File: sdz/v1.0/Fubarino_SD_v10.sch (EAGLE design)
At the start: 36 parts, among them IC1 PIC32MZXXXXECX064TQFP-10X10, IC2 MCP1702T-3302E/MB, IC3 DSC1033_MICREL_OSCILLATOR3.2X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, J1 MICRO_SD_CARD_SOCKET, J2 M28USEPIN1, J3 M28NOPIN1, J4 MICRO-USB-5P-340015001, Q2 32.768 KHz

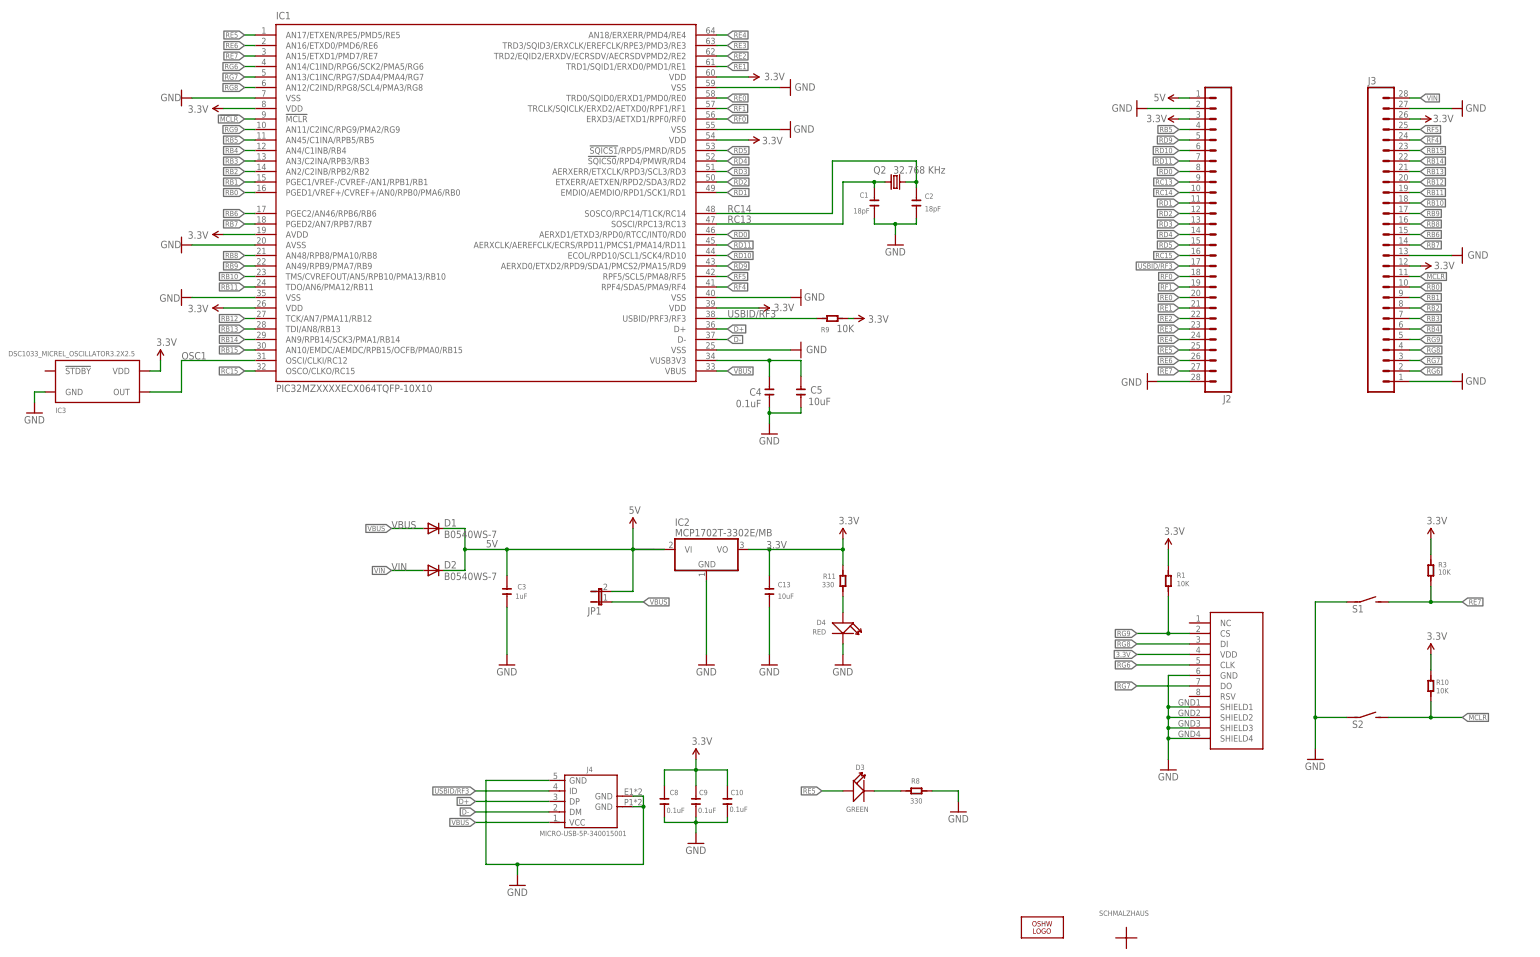
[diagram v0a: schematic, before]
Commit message: This version got sent to seed for fab - v 1.0
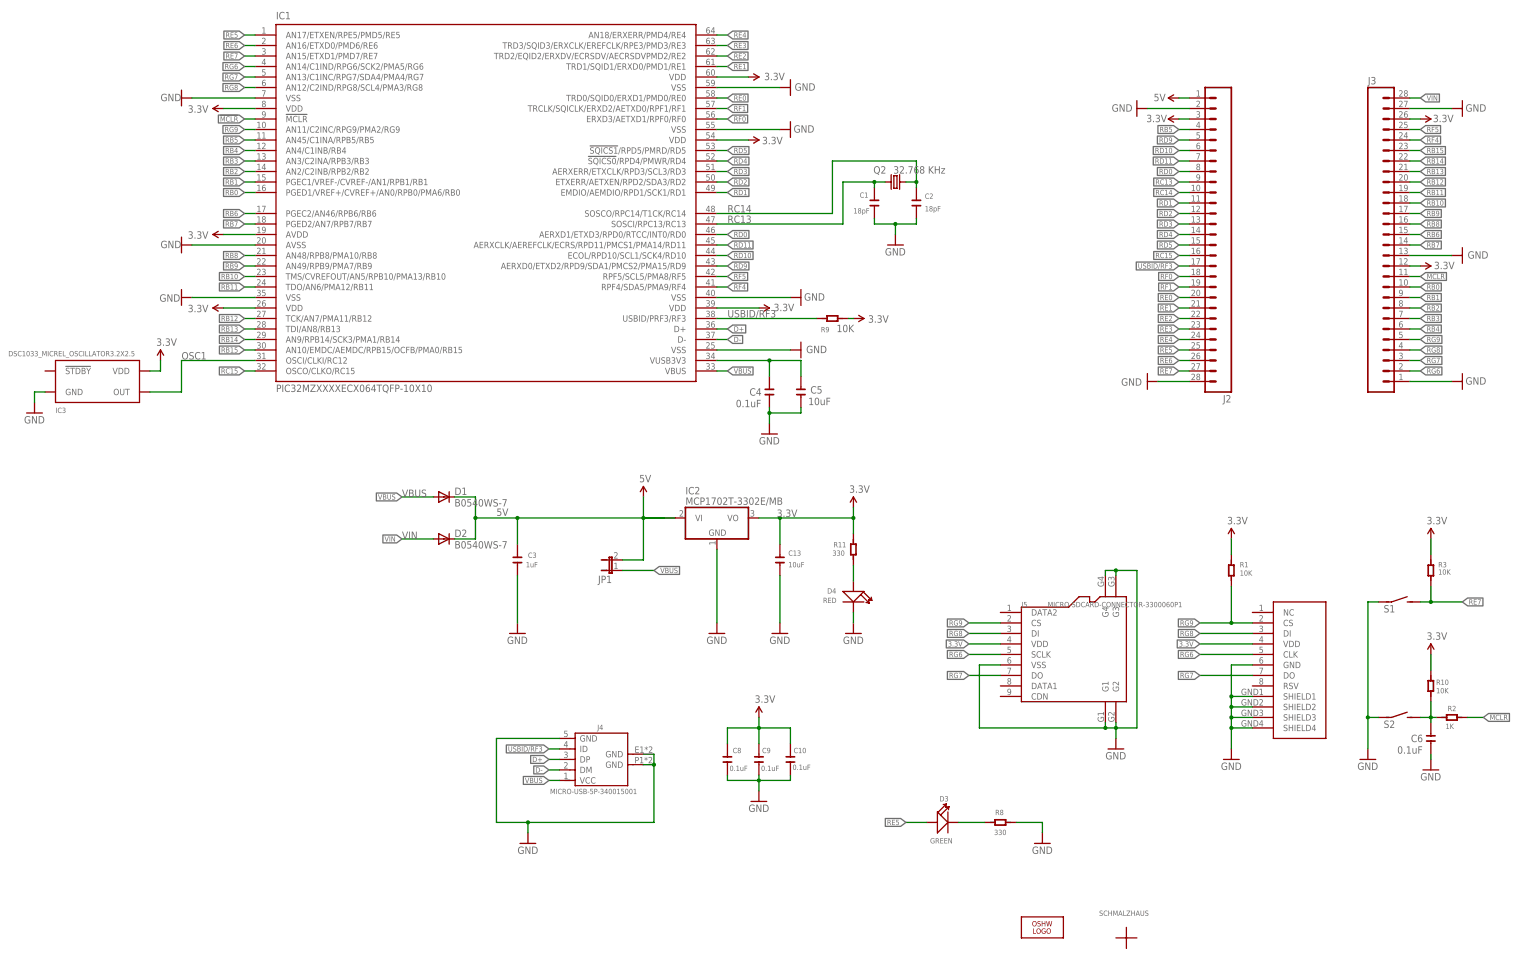
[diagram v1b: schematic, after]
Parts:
- added C6: 0.1uF, OPL Eagle Library:C-0603
- added J5: MICRO-SDCARD-CONNECTOR-3300060P1, OPL Eagle Library:MICRO-SDCARD-CONNECTOR-3300060P1
- added R2: 1K, OPL Eagle Library:R-0603
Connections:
- new net $MCLR: C6.1, R10.2, R2.1, S2.2
- net !MCLR!: now also R2.2; no longer R10.2, S2.2
- net 3.3V: now also J5.VDD
- net GND: now also C6.2, J5.G1, J5.G2, J5.G3, J5.G4, J5.VSS
- net RG6: now also J5.SCLK
- net RG7: now also J5.DO
- net RG8: now also J5.DI
- net RG9: now also J5.CS
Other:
- moved on the sheet: C10, C13, C3, C8, C9, D1, D2, D3, D4, IC2, J4, JP1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
